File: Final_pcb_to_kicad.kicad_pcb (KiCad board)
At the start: 2 copper layers, 3 parts, among them U1 CP_Radial_D10.0mm_P5.00mm, U2 C_Axial_L3.8mm_D2.6mm_P7.50mm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, U3 diplay_ali_16x2

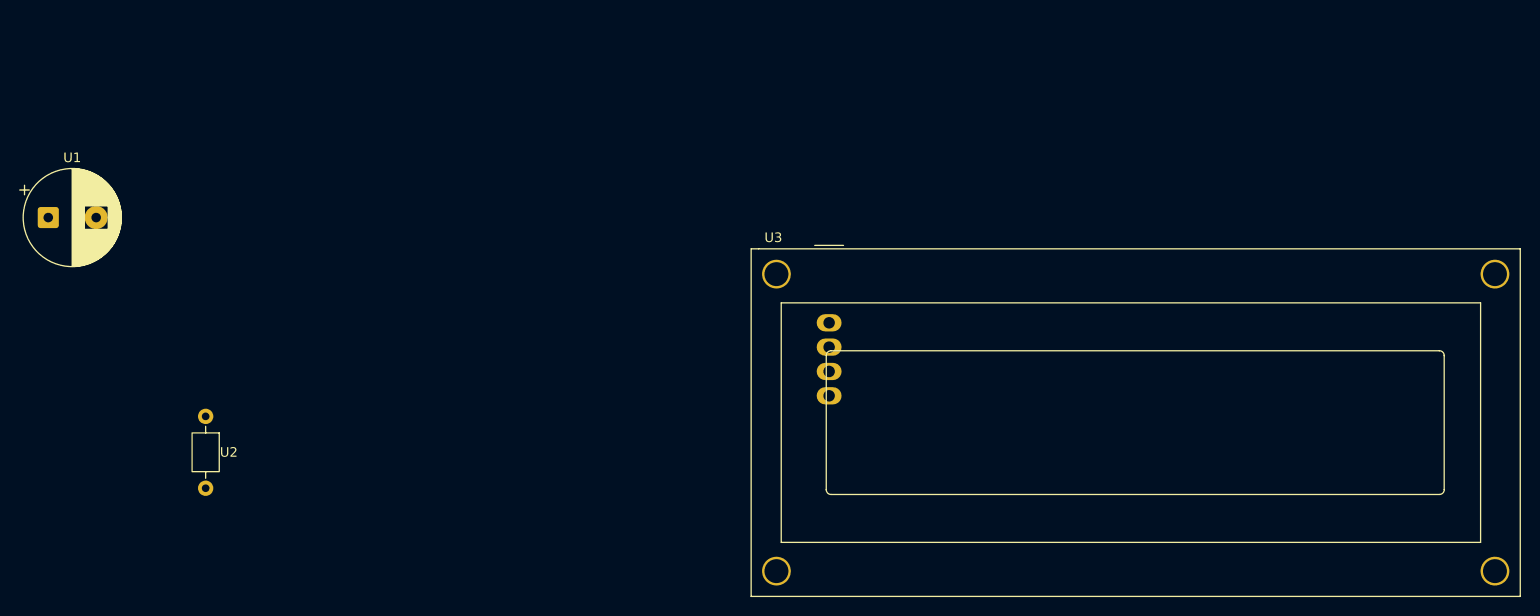
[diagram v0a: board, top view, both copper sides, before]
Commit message: backup - fix wire - nedokonceo
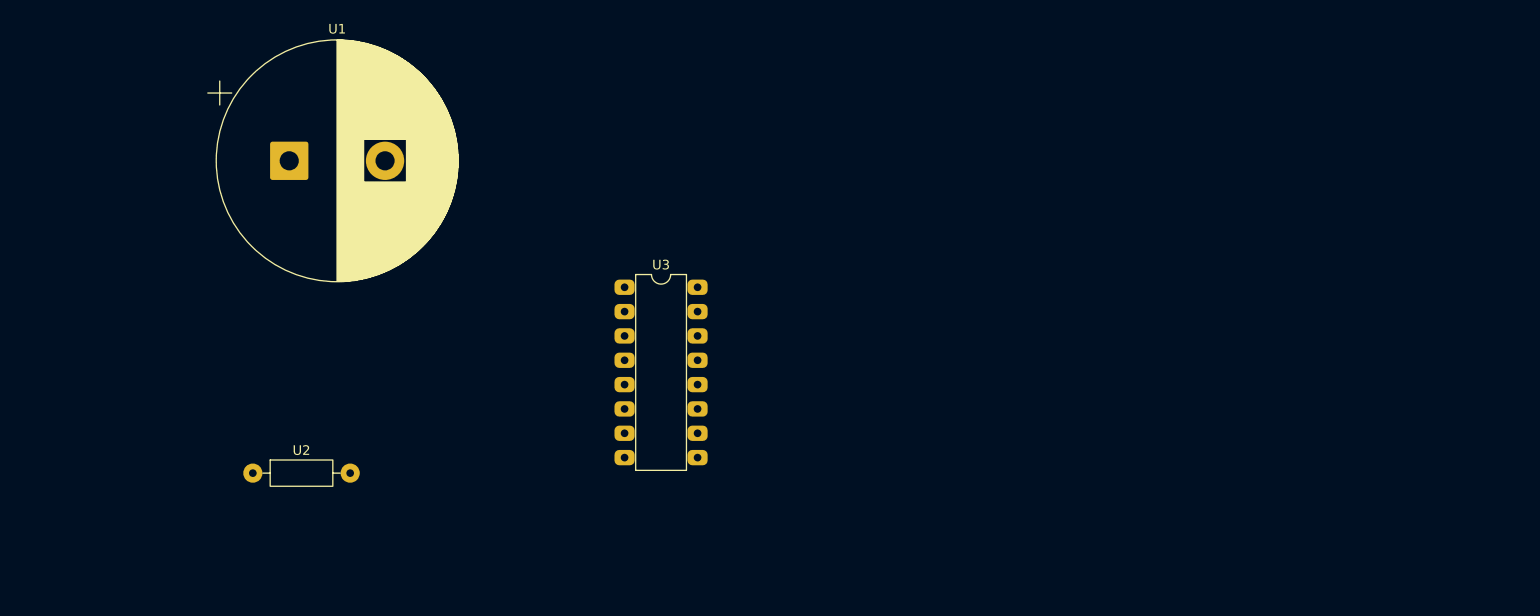
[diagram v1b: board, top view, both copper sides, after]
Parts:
- U1: value CP_Radial_D10.0mm_P5.00mm -> CP_Radial_D25.0mm_P10.00mm_SnapIn; footprint 00_basic:CP_Radial_D10.0mm_P5.00mm -> 00_basic:CP_Radial_D25.0mm_P10.00mm_SnapIn
- U2: value C_Axial_L3.8mm_D2.6mm_P7.50mm_Horizontal -> R_Axial_DIN0207_L6.3mm_D2.5mm_P10.16mm_Horizontal; footprint 00_basic:C_Axial_L3.8mm_D2.6mm_P7.50mm_Horizontal -> 00_basic:R_Axial_DIN0207_L6.3mm_D2.5mm_P10.16mm_Horizontal
- U3: value diplay_ali_16x2 -> DIP-16_W7.62mm; footprint 00_display:diplay_ali_16x2 -> 00_basic:DIP-16_W7.62mm
- moved U1 25.8 mm to (132.9, 88.7)
- moved U3 21.4 mm to (167.9, 101.9)
- moved U2 7.70 mm to (129.1, 121.3), turned to 0 degrees
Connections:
- U1 pad 1: Net_2 -> (no net)
- U1 pad 2: Net_1 -> (no net)
- U2 pad 1: Net_2 -> (no net)
- U2 pad 2: Net_1 -> (no net)
